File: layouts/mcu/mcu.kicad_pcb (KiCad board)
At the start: 2 copper layers, 12 parts

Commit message: Regenerate layouts
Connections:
- R2 pad 1: mcu-line-4 -> mcu-line-1
- R3 pad 2: mcu-line-8 -> mcu-line
- R4 pad 1: mcu-line-2 -> mcu-line-4
- R5 pad 1: mcu-line-5 -> mcu-line-6
- U1 pad 13: mcu-line-8 -> mcu-line
- U1 pad 16: mcu.esp32_c3_mini_1.ic-line-2 -> mcu.esp32_c3_mini_1.ic-line-3
- U1 pad 18: mcu.esp32_c3_mini_1.ic-line-5 -> mcu.esp32_c3_mini_1.ic-line-1
- U1 pad 19: mcu.esp32_c3_mini_1.ic-line-4 -> mcu.esp32_c3_mini_1.ic-line-5
- U1 pad 20: mcu.esp32_c3_mini_1.ic-line-3 -> mcu.esp32_c3_mini_1.ic-line-2
- U1 pad 21: mcu.esp32_c3_mini_1.ic-line -> mcu.esp32_c3_mini_1.ic-line-4
- U1 pad 22: mcu-line-5 -> mcu-line-6
- U1 pad 23: mcu-line-1 -> mcu-line-8
- U1 pad 26: mcu-line -> mcu-line-7
- U1 pad 30: mcu-line-7 -> mcu-line-5
- U1 pad 31: mcu-line-6 -> mcu-line-2
- U1 pad 5: mcu-line-2 -> mcu-line-4
- U1 pad 6: mcu.esp32_c3_mini_1.ic-line-1 -> mcu.esp32_c3_mini_1.ic-line
- U1 pad 8: mcu-line-4 -> mcu-line-1

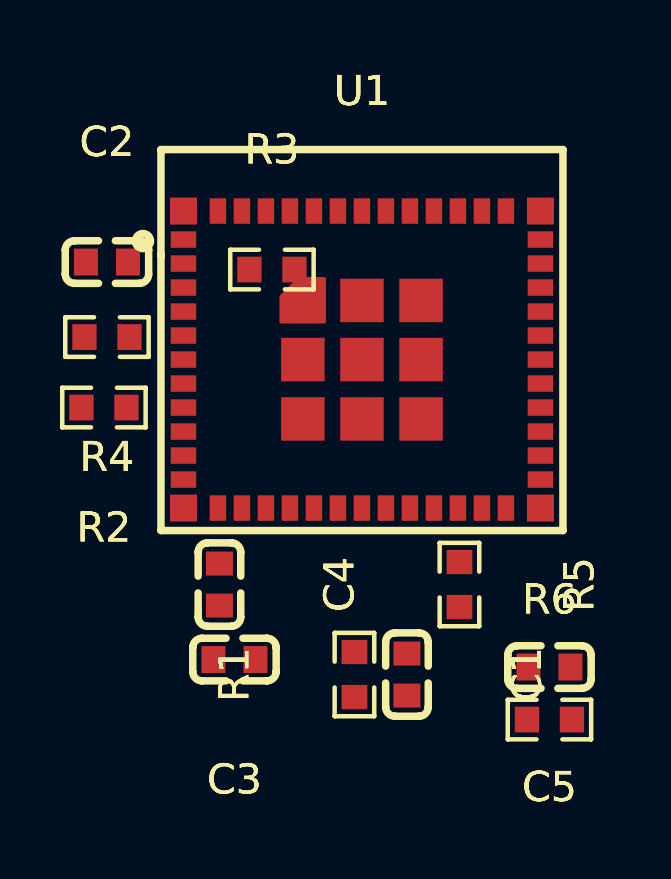
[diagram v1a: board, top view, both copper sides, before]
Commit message: Update layouts
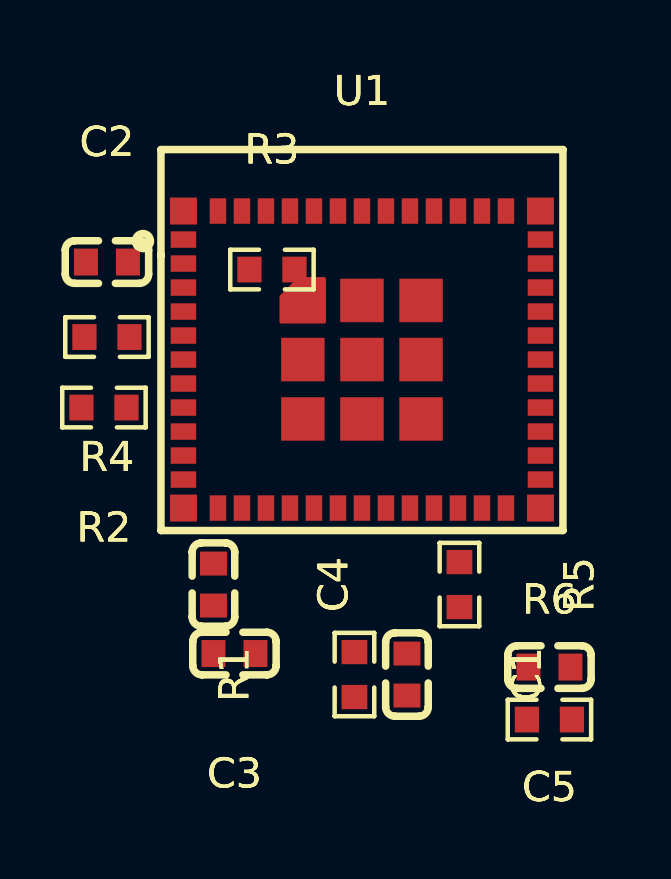
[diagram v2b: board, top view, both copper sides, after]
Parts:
- moved C4 0.20 mm to (-4.95, 7.50)
- moved C3 0.20 mm to (-4.25, 9.80)
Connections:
- C4 pad 1: mcu-line-9 -> mcu-line-2
- R2 pad 1: mcu-line-1 -> mcu-line-7
- R3 pad 2: mcu-line -> mcu-line-3
- R4 pad 1: mcu-line-4 -> mcu-line
- R5 pad 1: mcu-line-6 -> mcu-line-9
- U1 pad 12: mcu-line-9 -> mcu-line-2
- U1 pad 13: mcu-line -> mcu-line-3
- U1 pad 16: mcu.esp32_c3_mini_1.ic-line-3 -> mcu.esp32_c3_mini_1.ic-line-5
- U1 pad 19: mcu.esp32_c3_mini_1.ic-line-5 -> mcu.esp32_c3_mini_1.ic-line-2
- U1 pad 20: mcu.esp32_c3_mini_1.ic-line-2 -> mcu.esp32_c3_mini_1.ic-line-3
- U1 pad 22: mcu-line-6 -> mcu-line-9
- U1 pad 26: mcu-line-7 -> mcu-line-5
- U1 pad 27: mcu-line-3 -> mcu-line-6
- U1 pad 30: mcu-line-5 -> mcu-line-4
- U1 pad 31: mcu-line-2 -> mcu-line-1
- U1 pad 5: mcu-line-4 -> mcu-line
- U1 pad 8: mcu-line-1 -> mcu-line-7
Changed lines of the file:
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@@
             (outputdirectory "")))
     (net 0 "")
-    (net 1 "mcu-line-7")
+    (net 1 "mcu-line-5")
     (net 2 "mcu.esp32_c3_mini_1.ic.footprint.pins[26].net-net")
-    (net 3 "mcu-line-5")
+    (net 3 "mcu-line-4")
     (net 4 "mcu.esp32_c3_mini_1.ic.footprint.pins[8].net-net")
     (net 5 "mcu.esp32_c3_mini_1.ic.footprint.pins[28].net-net")
-    (net 6 "mcu.esp32_c3_mini_1.ic-line-5")
+    (net 6 "mcu.esp32_c3_mini_1.ic-line-2")
     (net 7 "mcu-line-8")
     (net 8 "mcu.esp32_c3_mini_1.ic.footprint.pins[25].net-net")
-    (net 9 "mcu-line-9")
-    (net 10 "mcu.esp32_c3_mini_1.ic-line-3")
-    (net 11 "mcu-line-3")
+    (net 9 "mcu-line-2")
+    (net 10 "mcu.esp32_c3_mini_1.ic-line-5")
+    (net 11 "mcu-line-6")
     (net 12 "mcu.esp32_c3_mini_1.ic.footprint.pins[60].net-net")
-    (net 13 "mcu-line-6")
+    (net 13 "mcu-line-9")
     (net 14 "mcu.boot_switch-line")
     (net 15 "mcu.low_speed_crystal_clock-net")
@@
     (net 17 "mcu.esp32_c3_mini_1.ic-line")
     (net 18 "mcu.esp32_c3_mini_1.ic.footprint.pins[16].net-net")
-    (net 19 "mcu-line-4")
+    (net 19 "mcu-line")
     (net 20 "mcu.esp32_c3_mini_1.ic.footprint.pins[58].net-net")
     (net 21 "mcu.esp32_c3_mini_1.ic.footprint.pins[21].net-net")
@@
     (net 25 "mcu.esp32_c3_mini_1.ic-line-4")
     (net 26 "hv")
-    (net 27 "mcu-line-2")
+    (net 27 "mcu-line-1")
     (net 28 "mcu.reset_switch.lp_filter-line")
     (net 29 "mcu.esp32_c3_mini_1.ic.footprint.pins[1].net-net")
-    (net 30 "mcu-line")
+    (net 30 "mcu-line-3")
     (net 31 "mcu.esp32_c3_mini_1.ic.footprint.pins[33].net-net")
     (net 32 "mcu.esp32_c3_mini_1.ic.footprint.pins[20].net-net")
     (net 33 "mcu.esp32_c3_mini_1.ic.footprint.pins[6].net-net")
     (net 34 "mcu-gnd")
-    (net 35 "mcu.esp32_c3_mini_1.ic-line-2")
+    (net 35 "mcu.esp32_c3_mini_1.ic-line-3")
     (net 36 "mcu.esp32_c3_mini_1.ic.footprint.pins[17].net-net")
     (net 37 "mcu.boot_switch.lp_filter-line")
     (net 38 "mcu.esp32_c3_mini_1.ic.footprint.pins[27].net-net")
-    (net 39 "mcu-line-1")
+    (net 39 "mcu-line-7")
     (footprint "atopile:R0603-ebcab9"
         (layer "F.Cu")
@@
     (footprint "atopile:C0603-bd72f6"
         (layer "F.Cu")
-        (at -4.25 10 180)
+        (at -4.25 9.8 180)
         (property "Reference" "C3"
             (at 0 -4 0)
@@
             (layers "F.Cu" "F.Paste" "F.Mask")
             (remove_unused_layers no)
-            (net 19 "mcu-line-4"))
+            (net 19 "mcu-line"))
         (pad "2" smd rect
             (at 0.75 0 180)
@@
             (layers "F.Cu" "F.Paste" "F.Mask")
             (remove_unused_layers no)
-            (net 39 "mcu-line-1"))
+            (net 39 "mcu-line-7"))
         (pad "2" smd rect
             (at 0.75 0 180)
@@
     (footprint "atopile:C0603-bd72f6"
         (layer "F.Cu")
-        (at -4.75 7.5 -90)
+        (at -4.95 7.5 -90)
         (property "Reference" "C4"
             (at 0 -4 90)
@@
             (layers "F.Cu" "F.Paste" "F.Mask")
             (remove_unused_layers no)
-            (net 9 "mcu-line-9"))
+            (net 9 "mcu-line-2"))
         (pad "2" smd rect
             (at 0.7 0 270)
@@
             (layers "F.Cu" "F.Paste" "F.Mask")
             (remove_unused_layers no)
-            (net 19 "mcu-line-4"))
+            (net 19 "mcu-line"))
         (pad "6" smd rect
             (at -5.95 0 0)
@@
             (layers "F.Cu" "F.Paste" "F.Mask")
             (remove_unused_layers no)
-            (net 39 "mcu-line-1"))
+            (net 39 "mcu-line-7"))
         (pad "9" smd rect
             (at -5.95 2.4 0)
@@
             (layers "F.Cu" "F.Paste" "F.Mask")
             (remove_unused_layers no)
-            (net 9 "mcu-line-9"))
+            (net 9 "mcu-line-2"))
         (pad "13" smd rect
             (at -4 4.95 90)
@@
             (layers "F.Cu" "F.Paste" "F.Mask")
             (remove_unused_layers no)
-            (net 30 "mcu-line"))
+            (net 30 "mcu-line-3"))
         (pad "14" smd rect
             (at -3.2 4.95 90)
@@
             (layers "F.Cu" "F.Paste" "F.Mask")
             (remove_unused_layers no)
-            (net 10 "mcu.esp32_c3_mini_1.ic-line-3"))
+            (net 10 "mcu.esp32_c3_mini_1.ic-line-5"))
         (pad "17" smd rect
             (at -0.8 4.95 90)
@@
             (layers "F.Cu" "F.Paste" "F.Mask")
             (remove_unused_layers no)
-            (net 6 "mcu.esp32_c3_mini_1.ic-line-5"))
+            (net 6 "mcu.esp32_c3_mini_1.ic-line-2"))
         (pad "20" smd rect
             (at 1.6 4.95 90)
@@
             (layers "F.Cu" "F.Paste" "F.Mask")
             (remove_unused_layers no)
-            (net 35 "mcu.esp32_c3_mini_1.ic-line-2"))
+            (net 35 "mcu.esp32_c3_mini_1.ic-line-3"))
         (pad "21" smd rect
             (at 2.4 4.95 90)
@@
             (layers "F.Cu" "F.Paste" "F.Mask")
             (remove_unused_layers no)
-            (net 13 "mcu-line-6"))
+            (net 13 "mcu-line-9"))
         (pad "23" smd rect
             (at 4 4.95 90)
@@
             (layers "F.Cu" "F.Paste" "F.Mask")
             (remove_unused_layers no)
-            (net 1 "mcu-line-7"))
+            (net 1 "mcu-line-5"))
         (pad "27" smd rect
             (at 5.95 2.4 180)
@@
             (layers "F.Cu" "F.Paste" "F.Mask")
             (remove_unused_layers no)
-            (net 11 "mcu-line-3"))
+            (net 11 "mcu-line-6"))
         (pad "28" smd rect
             (at 5.95 1.6 180)
@@
             (layers "F.Cu" "F.Paste" "F.Mask")
             (remove_unused_layers no)
-            (net 3 "mcu-line-5"))
+            (net 3 "mcu-line-4"))
         (pad "31" smd rect
             (at 5.95 -0.8 0)
@@
             (layers "F.Cu" "F.Paste" "F.Mask")
             (remove_unused_layers no)
-            (net 27 "mcu-line-2"))
+            (net 27 "mcu-line-1"))
         (pad "32" smd rect
             (at 5.95 -1.6 0)
@@
             (layers "F.Cu" "F.Paste" "F.Mask")
             (remove_unused_layers no)
-            (net 13 "mcu-line-6"))
+            (net 13 "mcu-line-9"))
         (pad "2" smd rect
             (at 0.75 0 270)
@@
         (attr smd)
         (fp_line
+            (start 1.39 -0.66)
+            (end 0.43 -0.66)
+            (stroke
+                (width 0.15)
+                (type solid))
+            (layer "F.SilkS")
+)
+        (fp_line
             (start -1.39 -0.66)
             (end -0.43 -0.66)
@@
 )
         (fp_line
+            (start 1.39 0.66)
+            (end 1.39 -0.66)
+            (stroke
+                (width 0.15)
+                (type solid))
+            (layer "F.SilkS")
+)
+        (fp_line
+            (start 0.43 0.66)
+            (end 1.39 0.66)
+            (stroke
+                (width 0.15)
+                (type solid))
+            (layer "F.SilkS")
+)
+        (fp_line
+            (start -0.43 0.66)
+            (end -1.39 0.66)
+            (stroke
+                (width 0.15)
+                (type solid))
+            (layer "F.SilkS")
+)
+        (fp_line
             (start -1.39 0.66)
             (end -1.39 -0.66)
-            (stroke
-                (width 0.15)
-                (type solid))
-            (layer "F.SilkS")
-)
-        (fp_line
-            (start -0.43 0.66)
-            (end -1.39 0.66)
-            (stroke
-                (width 0.15)
-                (type solid))
-            (layer "F.SilkS")
-)
-        (fp_line
-            (start 0.43 0.66)
-            (end 1.39 0.66)
-            (stroke
-                (width 0.15)
-                (type solid))
-            (layer "F.SilkS")
-)
-        (fp_line
-            (start 1.39 -0.66)
-            (end 0.43 -0.66)
-            (stroke
-                (width 0.15)
-                (type solid))
-            (layer "F.SilkS")
-)
-        (fp_line
-            (start 1.39 0.66)
-            (end 1.39 -0.66)
             (stroke
                 (width 0.15)
@@
             (unlocked no))
         (fp_text user "FBRK:autoplaced"
-            (at 0 0 0)
+            (at 0 -0.3 0)
             (layer "User.5")
             (effects
@@
             (layers "F.Cu" "F.Paste" "F.Mask")
             (remove_unused_layers no)
-            (net 30 "mcu-line"))))
+            (net 30 "mcu-line-3"))))
